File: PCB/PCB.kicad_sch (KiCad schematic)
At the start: 19 parts, among them J1 Conn_01x02_Pin, J10 Conn_01x02_Pin, J2 Conn_01x02_Pin, J3 Conn_01x02_Pin, J4 Conn_01x02_Pin, J5 Conn_01x02_Pin, J6 Conn_01x02_Pin, J7 Conn_01x02_Pin, J8 Conn_01x02_Pin, J9 Conn_01x04_Pin, U1 ESP32-WROOM-32E-N8R2

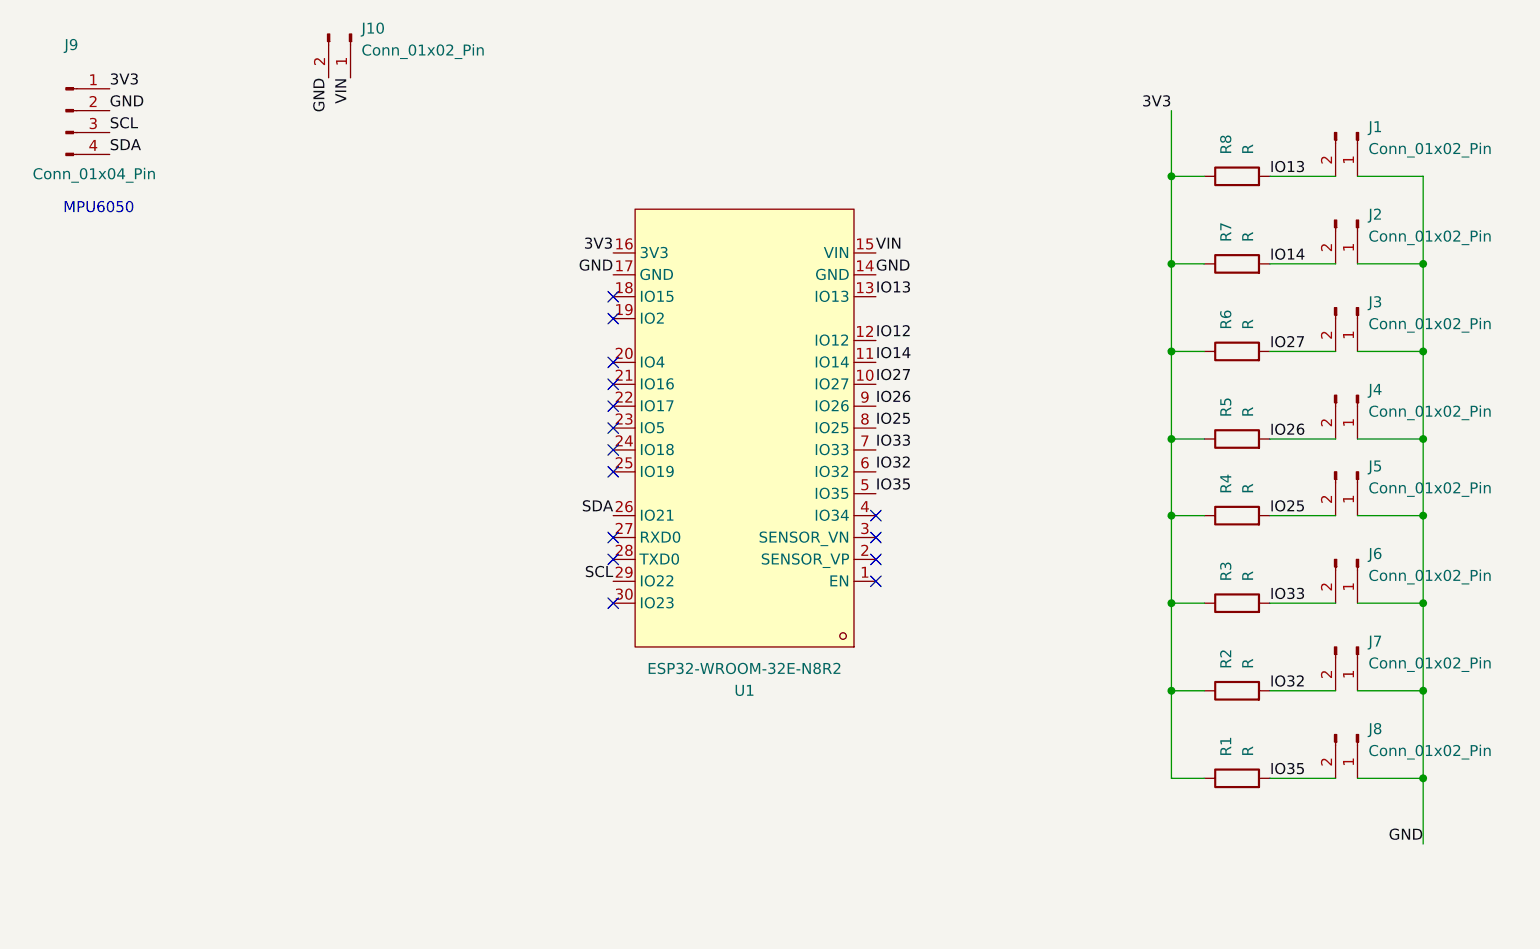
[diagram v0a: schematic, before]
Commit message: updates
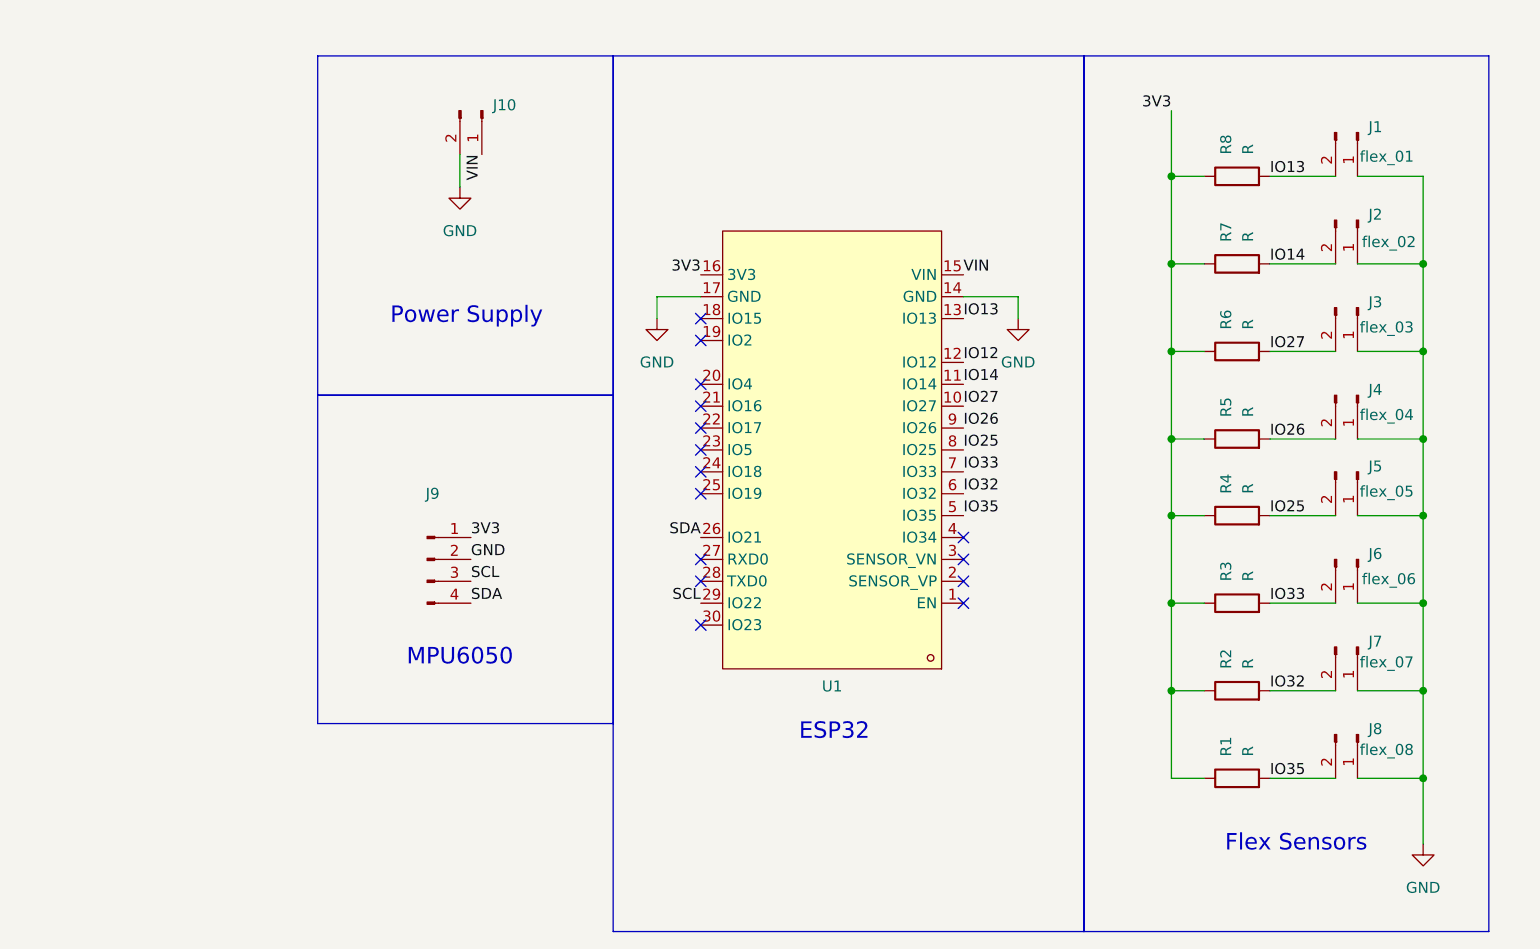
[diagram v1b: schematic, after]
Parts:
- J1: value Conn_01x02_Pin -> flex_01
- J2: value Conn_01x02_Pin -> flex_02
- J3: value Conn_01x02_Pin -> flex_03
- J4: value Conn_01x02_Pin -> flex_04
- J5: value Conn_01x02_Pin -> flex_05
- J6: value Conn_01x02_Pin -> flex_06
- J7: value Conn_01x02_Pin -> flex_07
- J8: value Conn_01x02_Pin -> flex_08
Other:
- note added: "ESP32"
- note added: "Flex Sensors"
- note added: "Power Supply"
- moved on the sheet: J10, J9, U1
